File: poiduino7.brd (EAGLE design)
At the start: 67.8 x 53.4 mm, 20 parts, among them K1 TS-1109, Y1 16MHZ

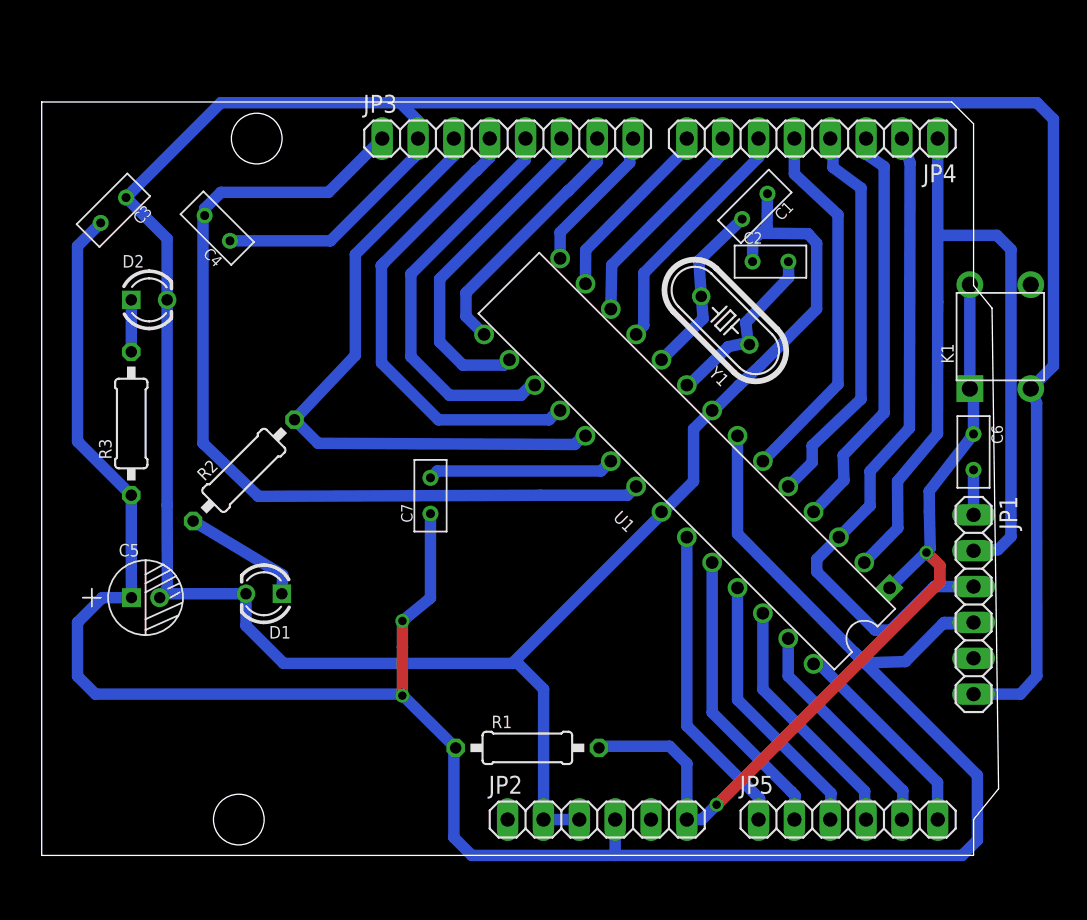
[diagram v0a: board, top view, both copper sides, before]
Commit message: new board
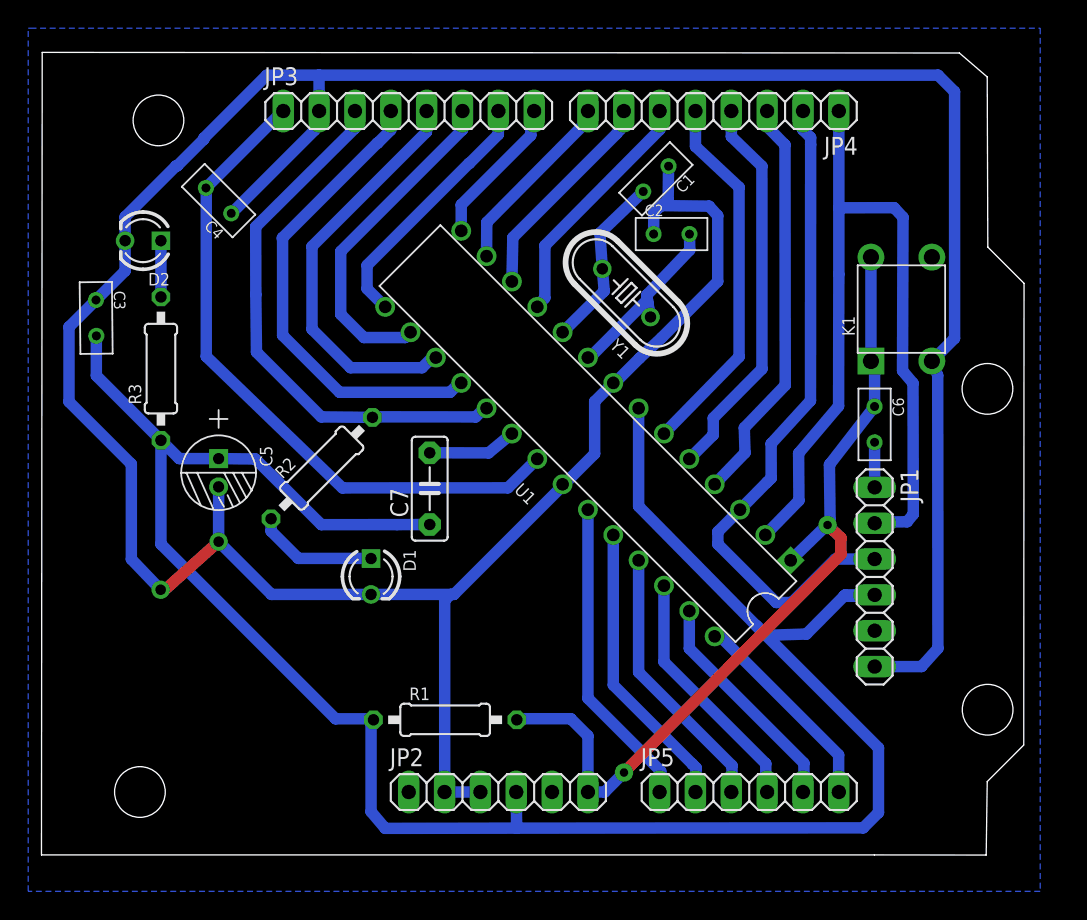
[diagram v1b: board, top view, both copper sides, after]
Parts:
- C7: device Seeed-Capacitor:CERAMIC-2.54 -> capacitor-wima:C5B2.5
- moved C5 10.3 mm to (12.5, 27.1), turned to 270 degrees
- moved C3 7.73 mm to (3.86, 38.1), turned to 270.6 degrees
- moved D1 7.69 mm to (23.3, 19.8), turned to 270 degrees
- moved JP1 7.28 mm to (59.0, 19.7)
- moved JP3 7.28 mm to (26.0, 52.8)
- moved C1 7.28 mm to (43.5, 47.9)
- moved JP4 7.28 mm to (47.6, 52.8)
- moved JP2 7.28 mm to (32.4, 4.49)
- moved JP5 7.28 mm to (50.1, 4.49)
- moved C2 7.28 mm to (44.6, 44.0)
- moved K1 7.28 mm to (60.9, 38.7)
- moved U1 7.28 mm to (38.7, 29.9)
- moved Y1 7.28 mm to (41.4, 39.9)
- moved C6 7.28 mm to (59.0, 30.5)
- moved R1 6.16 mm to (28.5, 9.61)
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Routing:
- net VCC: track 176.4 -> 153.8 mm, vias 2 -> 0
- net AREF: track 63.8 -> 47.8 mm
- net GND: track 256.4 -> 241.4 mm, vias 0 -> 2
- net PIN13: track 46.1 -> 38.6 mm
- net AVCC: track 13.3 -> 6.32 mm
- net XTAL1: track 12.7 -> 14.3 mm
- net RESET: track 62.1 -> 60.9 mm
- added copper zone on layer 16, net GND
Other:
- board size 67.8 x 53.4 mm -> 69.6 x 56.9 mm
